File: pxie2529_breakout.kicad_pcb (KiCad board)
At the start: 2 copper layers, 1 part, among them J1 connector-25x4

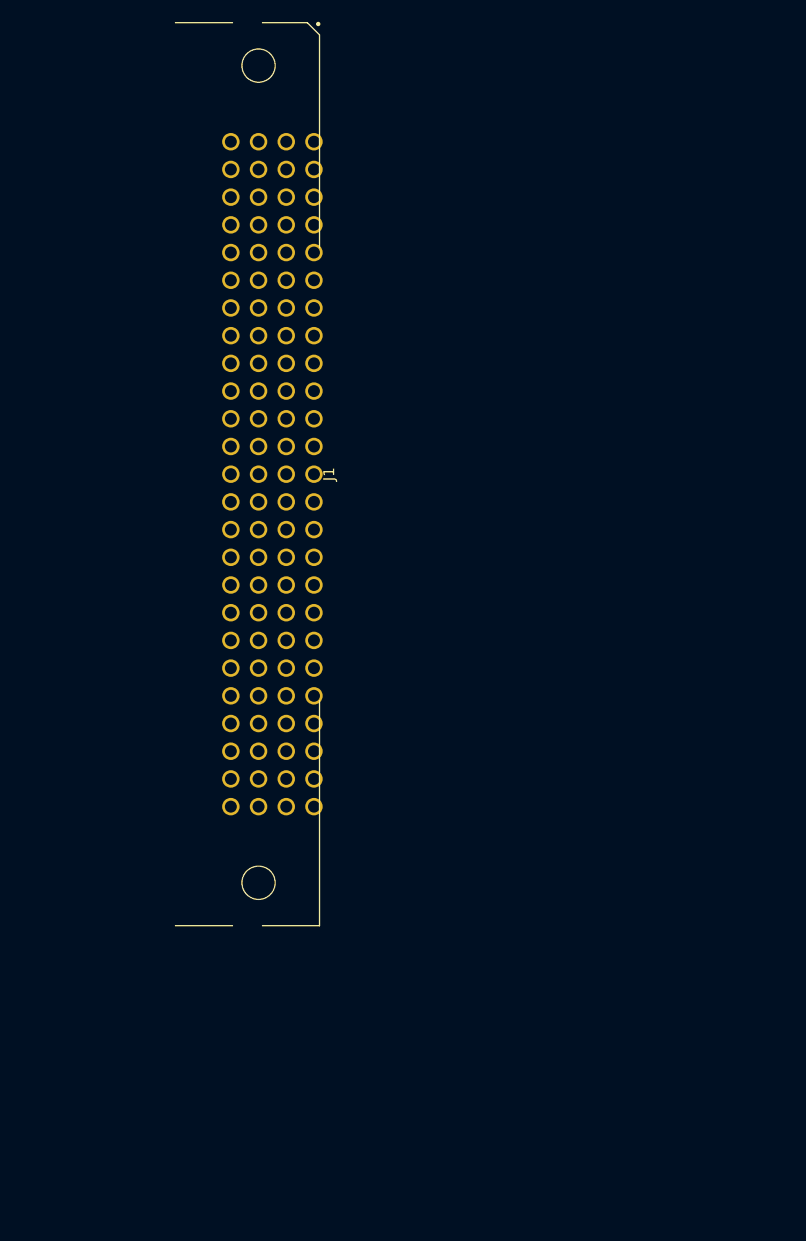
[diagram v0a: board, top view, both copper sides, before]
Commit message: finished routing
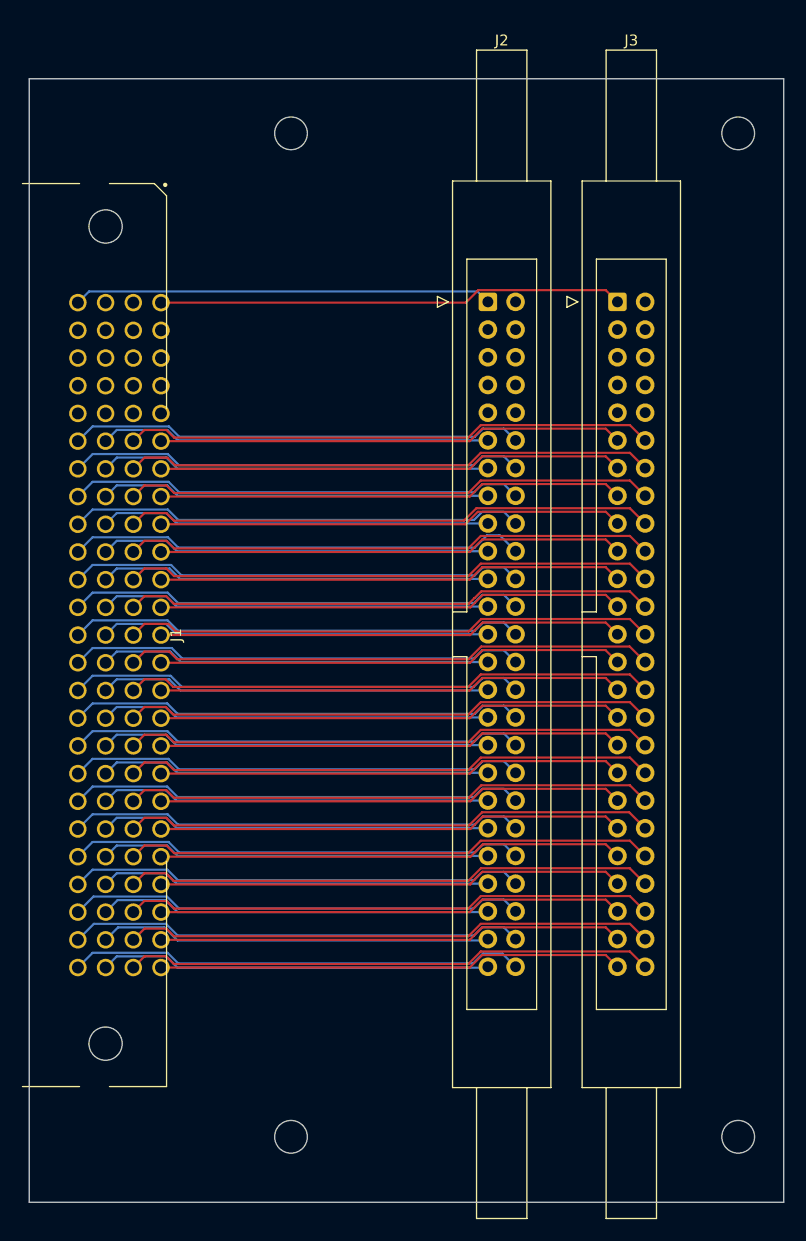
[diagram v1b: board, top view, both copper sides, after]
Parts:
- added J2: Conn_02x25_Odd_Even, Connector_IDC:IDC-Header_2x25_P2.54mm_Latch12.0mm_Vertical, F.Cu at (102.0, 78.5)
- added J3: Conn_02x25_Odd_Even, Connector_IDC:IDC-Header_2x25_P2.54mm_Latch12.0mm_Vertical, F.Cu at (113.9, 78.5)
- moved J1 20.4 mm to (67.0, 109.0)
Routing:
- net /B0R2+: track 0.00 -> 48.8 mm
- net /B1C0+: track 0.00 -> 48.7 mm
- net /B0C2+: track 0.00 -> 48.7 mm
- net /B1C2+: track 0.00 -> 48.7 mm
- net /B1R0+: track 0.00 -> 48.7 mm
- net /B1C9+: track 0.00 -> 48.7 mm
- net /B1C11+: track 0.00 -> 48.7 mm
- net /B0R0+: track 0.00 -> 48.7 mm
- net /B0C0+: track 0.00 -> 48.7 mm
- net /B0C10+: track 0.00 -> 48.7 mm
- net /B1C1+: track 0.00 -> 48.7 mm
- net /B1R2+: track 0.00 -> 48.7 mm
- net /B0C8+: track 0.00 -> 48.7 mm
- net /B1C8+: track 0.00 -> 48.7 mm
- net /B1C3+: track 0.00 -> 48.7 mm
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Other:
- board outline added: 69.2 x 103 mm
- net class Default: clearance 0.2 -> 0.125; trace_width 0.25 -> 0.2; via_dia 0.8 -> 0.6; via_drill 0.4 -> 0.3
- rule trace_clearance: 0.2 -> 0.125
- rule trace_min: 0.2 -> 0.125
- rule via_min_size: 0.4 -> 0.6
